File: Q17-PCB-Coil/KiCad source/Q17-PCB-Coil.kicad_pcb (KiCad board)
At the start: 2 copper layers, 35 x 39 mm, 3 parts, among them J1-1 INPUT, J1-2 OUTPUT

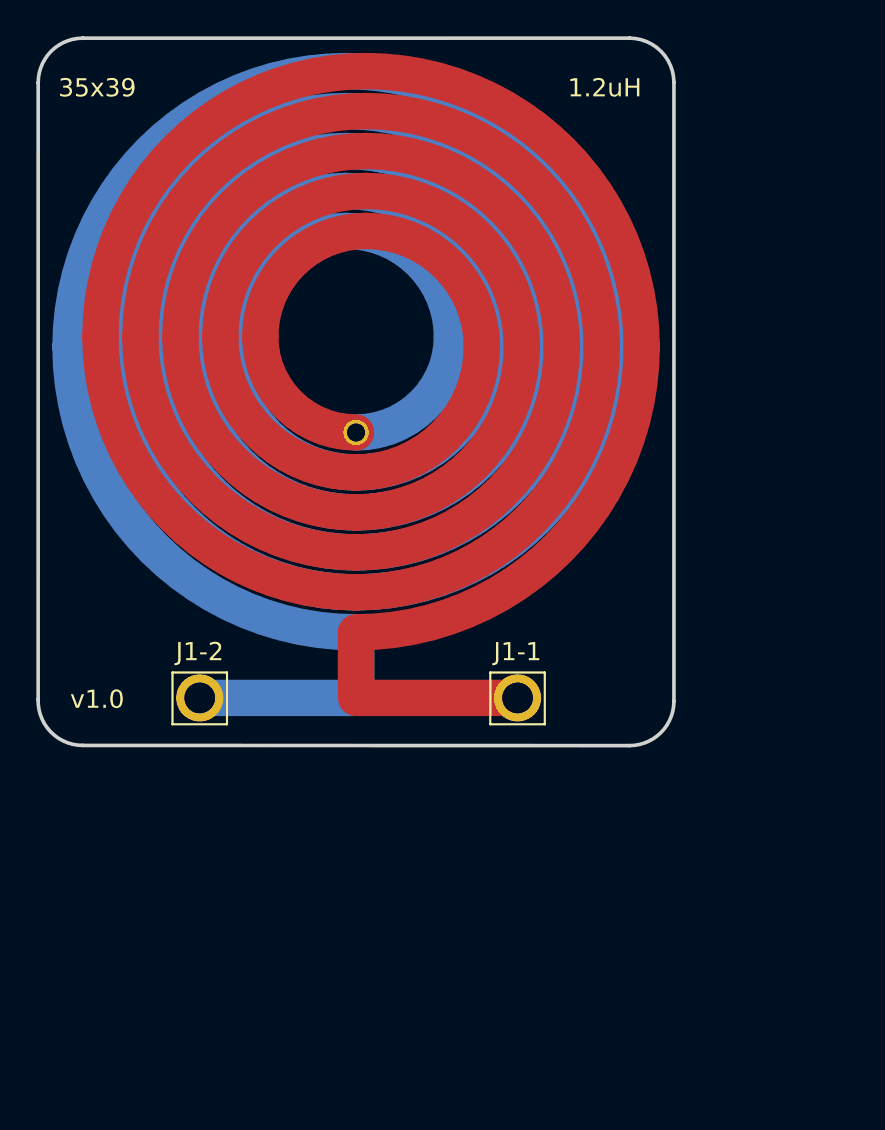
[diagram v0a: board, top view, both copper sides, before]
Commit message: Update Gerber-Q17-PCB-Coil-1.0
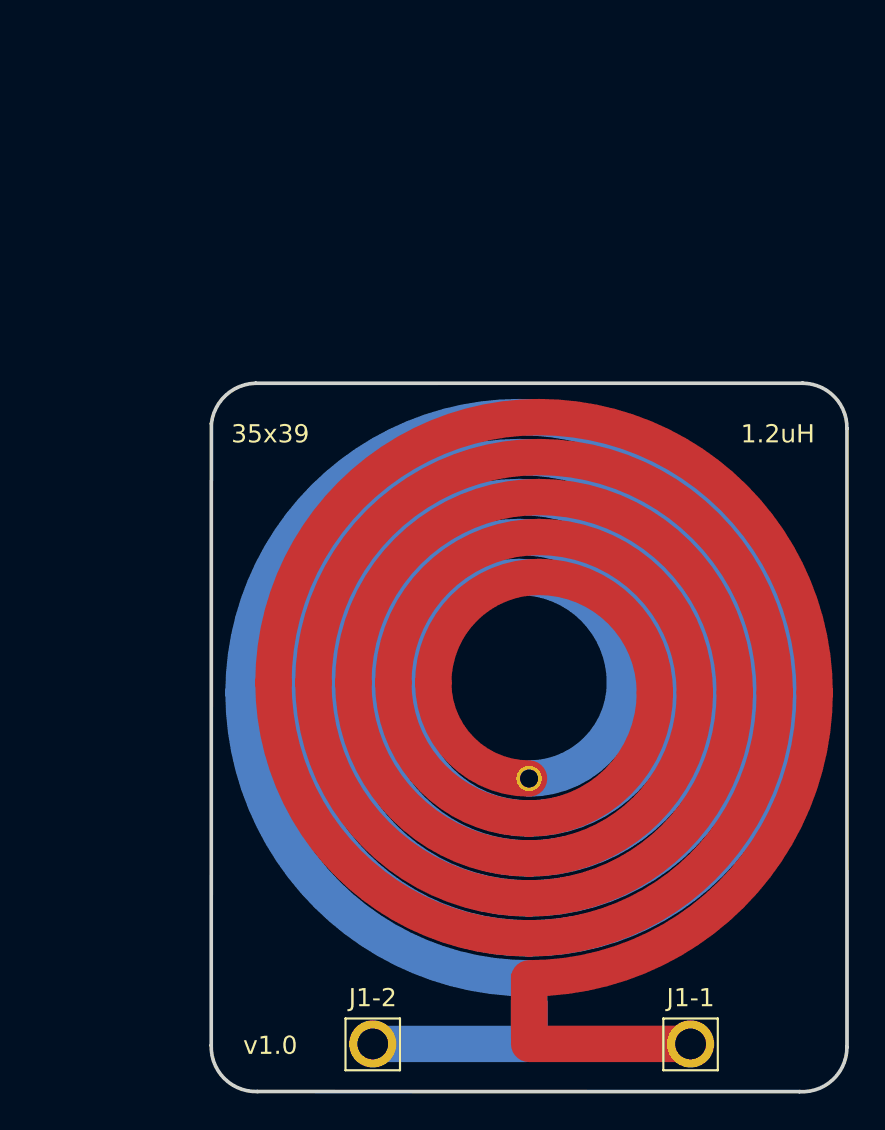
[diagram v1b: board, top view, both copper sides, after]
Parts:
- moved J1-1 21.3 mm to (158.4, 105.3)
- moved J1-2 21.3 mm to (140.9, 105.3)
- moved L1 21.3 mm to (149.5, 85.7)
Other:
- outline, holes or cut-outs redrawn
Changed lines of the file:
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@@
   (title_block
     (title "Q17 1.2uH inductor")
-    (date "2021-12-31")
+    (date "2022-01-01")
     (rev "1.0")
     (company "PCB design by Stef")
@@
   (net 2 "Net-(L1-Pad2)")
   (footprint "Connector_Pin:Pin_D1.4mm_L8.5mm_W2.8mm_FlatFork" (layer "F.Cu")
-    (at 131.37286 86.277667)
+    (at 140.89786 105.327667)
     (descr "solder Pin_ with flat with fork, hole diameter 1.4mm, length 8.5mm, width 2.8mm, e.g. Ettinger 13.13.890, https://katalog.ettinger.de/#p=434")
     (tags "solder Pin_ with flat fork")
@@
   )
   (footprint "Q17_Library:L_new" (layer "F.Cu")
-    (at 139.979941 66.664933 -90)
+    (at 149.504941 85.714933 -90)
     (descr "spiral inductor")
     (tags "SMD")
@@
   )
   (footprint "Connector_Pin:Pin_D1.4mm_L8.5mm_W2.8mm_FlatFork" (layer "F.Cu")
-    (at 148.87 86.277667)
+    (at 158.395 105.327667)
     (descr "solder Pin_ with flat with fork, hole diameter 1.4mm, length 8.5mm, width 2.8mm, e.g. Ettinger 13.13.890, https://katalog.ettinger.de/#p=434")
     (tags "solder Pin_ with flat fork")
@@
     )
   )
-  (gr_line (start 157.478892 52.402157) (end 157.480591 86.453795) (layer "Edge.Cuts") (width 0.2))
-  (gr_arc (start 122.477074 52.403333) (mid 123.194662 50.670922) (end 124.927073 49.953334) (layer "Edge.Cuts") (width 0.2))
-  (gr_arc (start 157.480591 86.453795) (mid 156.763003 88.186206) (end 155.030592 88.903794) (layer "Edge.Cuts") (width 0.2))
-  (gr_arc (start 155.039003 49.952159) (mid 156.764947 50.673278) (end 157.479003 52.402157) (layer "Edge.Cuts") (width 0.2))
-  (gr_line (start 124.927073 49.953334) (end 155.039003 49.952159) (layer "Edge.Cuts") (width 0.2))
-  (gr_arc (start 124.93042 88.892152) (mid 123.166833 88.145713) (end 122.474997 86.36) (layer "Edge.Cuts") (width 0.2))
-  (gr_line (start 124.93042 88.892152) (end 155.030592 88.903794) (layer "Edge.Cuts") (width 0.2))
-  (gr_line (start 122.477074 52.403333) (end 122.474997 86.36) (layer "Edge.Cuts") (width 0.2))
-  (gr_line (start 157.248072 52.588014) (end 157.242529 86.304428) (layer "Margin") (width 0.2))
-  (gr_line (start 125.153851 50.159163) (end 154.890169 50.132998) (layer "Margin") (width 0.2))
-  (gr_line (start 122.672407 52.415663) (end 122.685584 86.455378) (layer "Margin") (width 0.2))
-  (gr_arc (start 125.142299 88.694282) (mid 123.425217 88.1111) (end 122.685584 86.455378) (layer "Margin") (width 0.2))
-  (gr_arc (start 154.890169 50.132998) (mid 156.617594 50.833728) (end 157.248072 52.588014) (layer "Margin") (width 0.2))
-  (gr_line (start 125.142299 88.694282) (end 154.914815 88.689783) (layer "Margin") (width 0.2))
-  (gr_arc (start 122.666854 52.43804) (mid 123.408811 50.751256) (end 125.153851 50.159163) (layer "Margin") (width 0.2))
-  (gr_arc (start 157.242529 86.304428) (mid 156.612365 88.017902) (end 154.914815 88.689783) (layer "Margin") (width 0.2))
-  (gr_rect locked (start 122.48 49.9) (end 157.48 88.9) (layer "User.4") (width 0.015) (fill none))
-  (gr_text "1.2uH" (at 153.67 52.694933) (layer "F.SilkS")
+  (gr_line (start 167.003892 71.452157) (end 167.005591 105.503795) (layer "Edge.Cuts") (width 0.2))
+  (gr_arc (start 132.01208 71.189443) (mid 132.810124 69.610666) (end 134.452073 68.952324) (layer "Edge.Cuts") (width 0.2))
+  (gr_arc (start 167.005591 105.503795) (mid 166.228817 107.295707) (end 164.39 107.953794) (layer "Edge.Cuts") (width 0.2))
+  (gr_line (start 134.545 107.947943) (end 164.39 107.953794) (layer "Edge.Cuts") (width 0.2))
+  (gr_arc (start 164.564003 68.951149) (mid 166.307998 69.690409) (end 167.003892 71.452157) (layer "Edge.Cuts") (width 0.2))
+  (gr_line (start 134.452073 68.952324) (end 164.564003 68.951149) (layer "Edge.Cuts") (width 0.2))
+  (gr_arc (start 134.545 107.947943) (mid 132.724964 107.230249) (end 132.005 105.41111) (layer "Edge.Cuts") (width 0.2))
+  (gr_line (start 132.01208 71.189443) (end 132.005 105.41111) (layer "Edge.Cuts") (width 0.2))
+  (gr_line (start 166.773072 71.638014) (end 166.767529 105.354428) (layer "Margin") (width 0.2))
+  (gr_line (start 134.678851 69.209163) (end 164.415169 69.182998) (layer "Margin") (width 0.2))
+  (gr_line (start 132.197407 71.465663) (end 132.210584 105.505378) (layer "Margin") (width 0.2))
+  (gr_arc (start 134.667299 107.744282) (mid 132.950217 107.1611) (end 132.210584 105.505378) (layer "Margin") (width 0.2))
+  (gr_arc (start 164.415169 69.182998) (mid 166.133218 69.892734) (end 166.773072 71.638014) (layer "Margin") (width 0.2))
+  (gr_line (start 134.667299 107.744282) (end 164.439815 107.739783) (layer "Margin") (width 0.2))
+  (gr_arc (start 132.191854 71.48804) (mid 132.933811 69.801256) (end 134.678851 69.209163) (layer "Margin") (width 0.2))
+  (gr_arc (start 166.767529 105.354428) (mid 166.120332 107.051281) (end 164.439815 107.739783) (layer "Margin") (width 0.2))
+  (gr_rect locked (start 132.005 68.95) (end 167.005 107.95) (layer "User.4") (width 0.2) (fill none))
+  (gr_text "1.2uH" (at 163.195 71.744933) (layer "F.SilkS")
     (effects (font (size 1 1) (thickness 0.15)))
   )
-  (gr_text "v1.0" (at 125.73 86.36) (layer "F.SilkS")
+  (gr_text "v1.0" (at 135.255 105.41) (layer "F.SilkS")
     (effects (font (size 1 1) (thickness 0.15)))
   )
-  (gr_text "35x39" (at 125.73 52.694933) (layer "F.SilkS")
+  (gr_text "35x39" (at 135.255 71.744933) (layer "F.SilkS")
     (effects (font (size 1 1) (thickness 0.15)))
   )
-  (segment (start 139.98 86.277667) (end 148.702734 86.277667) (width 2) (layer "F.Cu") (net 1))
-  (segment (start 139.98 83.904933) (end 139.98 85.927675) (width 2) (layer "F.Cu") (net 1))
-  (segment (start 131.37286 86.277667) (end 139.797333 86.277667) (width 2) (layer "B.Cu") (net 2))
-  (segment (start 139.797333 86.277667) (end 139.98 86.095) (width 0.25) (layer "B.Cu") (net 2))
-  (segment (start 139.979941 86.094941) (end 139.979941 83.904933) (width 2) (layer "B.Cu") (net 2))
-  (segment (start 139.98 86.095) (end 139.979941 86.094941) (width 2) (layer "B.Cu") (net 2))
+  (segment (start 149.505 105.327667) (end 158.227734 105.327667) (width 2) (layer "F.Cu") (net 1))
+  (segment (start 149.505 102.954933) (end 149.505 104.977675) (width 2) (layer "F.Cu") (net 1))
+  (segment (start 140.89786 105.327667) (end 149.322333 105.327667) (width 2) (layer "B.Cu") (net 2))
+  (segment (start 149.322333 105.327667) (end 149.505 105.145) (width 0.25) (layer "B.Cu") (net 2))
+  (segment (start 149.504941 105.144941) (end 149.504941 102.954933) (width 2) (layer "B.Cu") (net 2))
+  (segment (start 149.505 105.145) (end 149.504941 105.144941) (width 2) (layer "B.Cu") (net 2))
 )
